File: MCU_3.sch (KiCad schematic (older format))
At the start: 18 parts, among them U2 STM32F051K6Ux

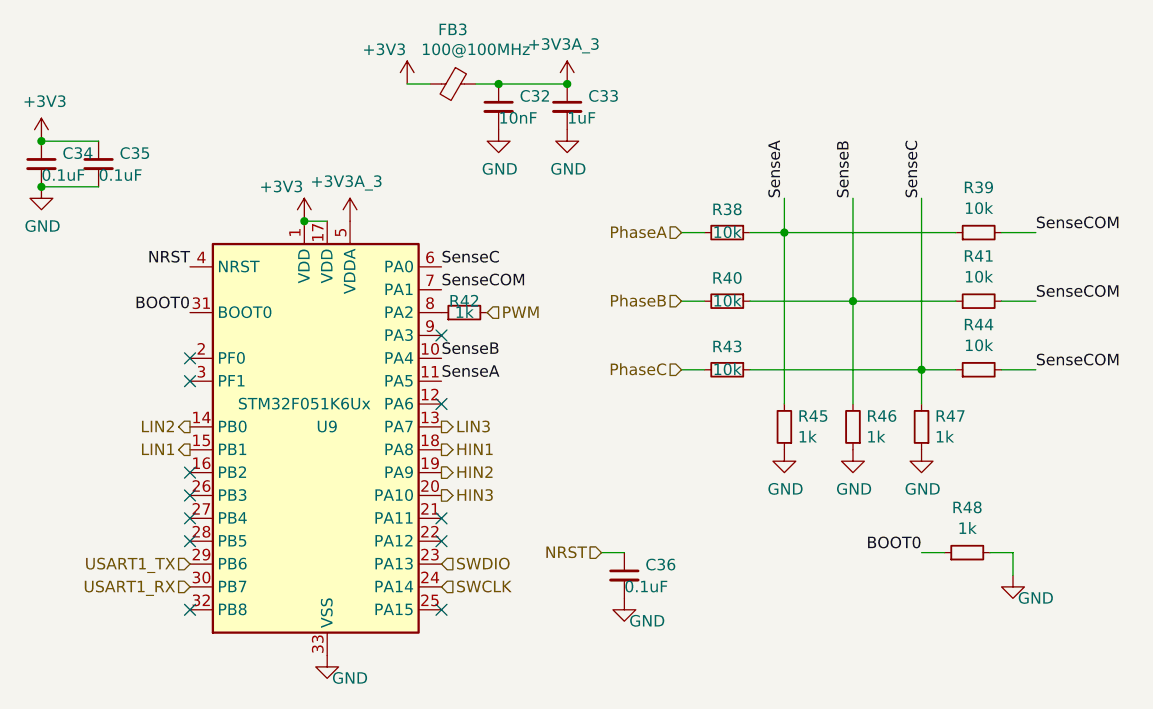
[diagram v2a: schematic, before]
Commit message: Added stuff
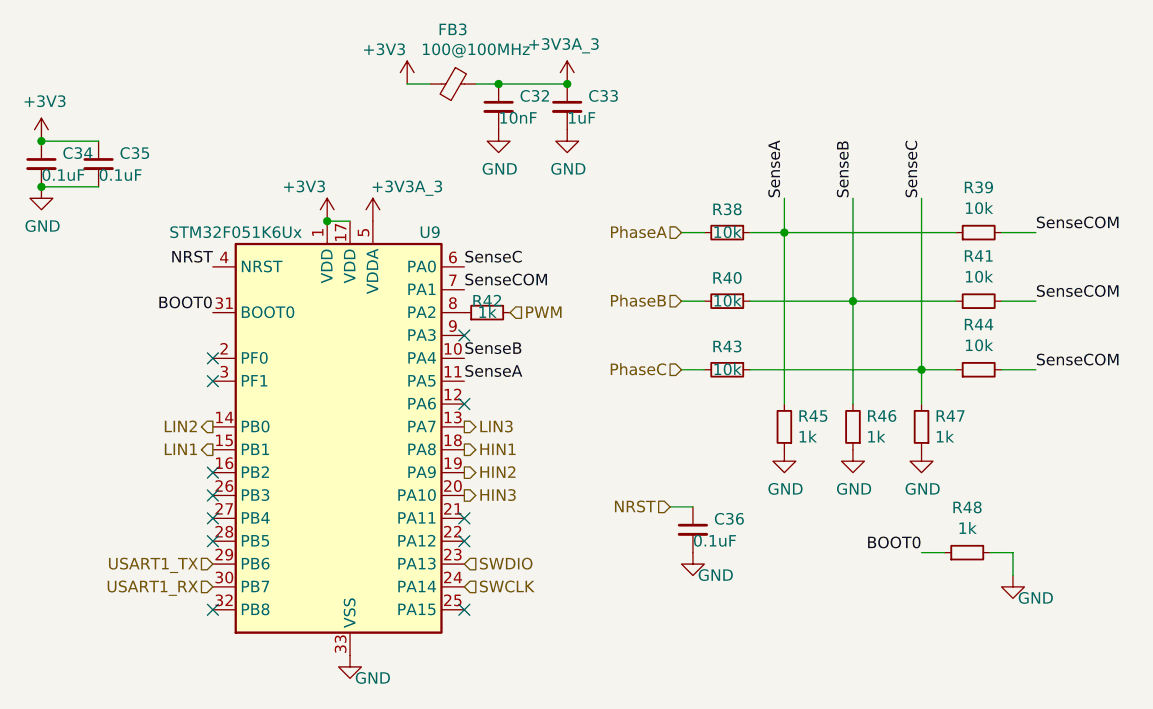
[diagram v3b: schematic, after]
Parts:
- removed U2: STM32F051K6Ux, Package_DFN_QFN:QFN-32-1EP_5x5mm_P0.5mm_EP3.45x3.45mm, symbol MCU_ST_STM32F0:STM32F051K6Ux
- added U9: STM32F051K6Ux, Package_DFN_QFN:QFN-32-1EP_5x5mm_P0.5mm_EP3.45x3.45mm, symbol MCU_ST_STM32F0:STM32F051K6Ux
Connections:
- net +3.3VA_3: now also U9.5 (VDDA)
- net +3V3: now also U9.1 (VDD), U9.17 (VDD)
- net BOOT0: now also U9.31 (BOOT0)
- net GND: now also U9.33 (VSS)
- net HIN1: now also U9.18 (PA8)
- net HIN2: now also U9.19 (PA9)
- net HIN3: now also U9.20 (PA10)
- net LIN1: now also U9.15 (PB1)
- net LIN2: now also U9.14 (PB0)
- net LIN3: now also U9.13 (PA7)
- net NRST: now also U9.4 (NRST)
- net SWCLK: now also U9.24 (PA14)
- net SWDIO: now also U9.23 (PA13)
- net SenseA: now also U9.11 (PA5)
- net SenseB: now also U9.10 (PA4)
- net SenseC: now also U9.6 (PA0)
- net SenseCOM: now also U9.7 (PA1)
- net USART1_RX: now also U9.30 (PB7)
- net USART1_TX: now also U9.29 (PB6)
- net at R24.1: now also U9.8 (PA2)
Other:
- moved on the sheet: C36, R42
